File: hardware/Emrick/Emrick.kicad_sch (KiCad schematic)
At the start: 85 parts, among them J1 LED_STRIP_CONNECTOR, J2 UFL, J3 Conn_02x05_Odd_Even, J4 BATT_CONN, P1 USB_C_Plug_USB2.0, Q1 Q_NPN_DGS, Q2 Q_NPN_DGS, Q3 Q_NPN_DGS, SW1 SW_SPST, SW2 SW_MEC_5E (RESET), U1 74HCT541, U2 CC1310, U3 TPS63020, U4 CP2102N, U5 MX25R8035F, U6 BQ24072, Y1 24MHz, Y2 32.768kHz

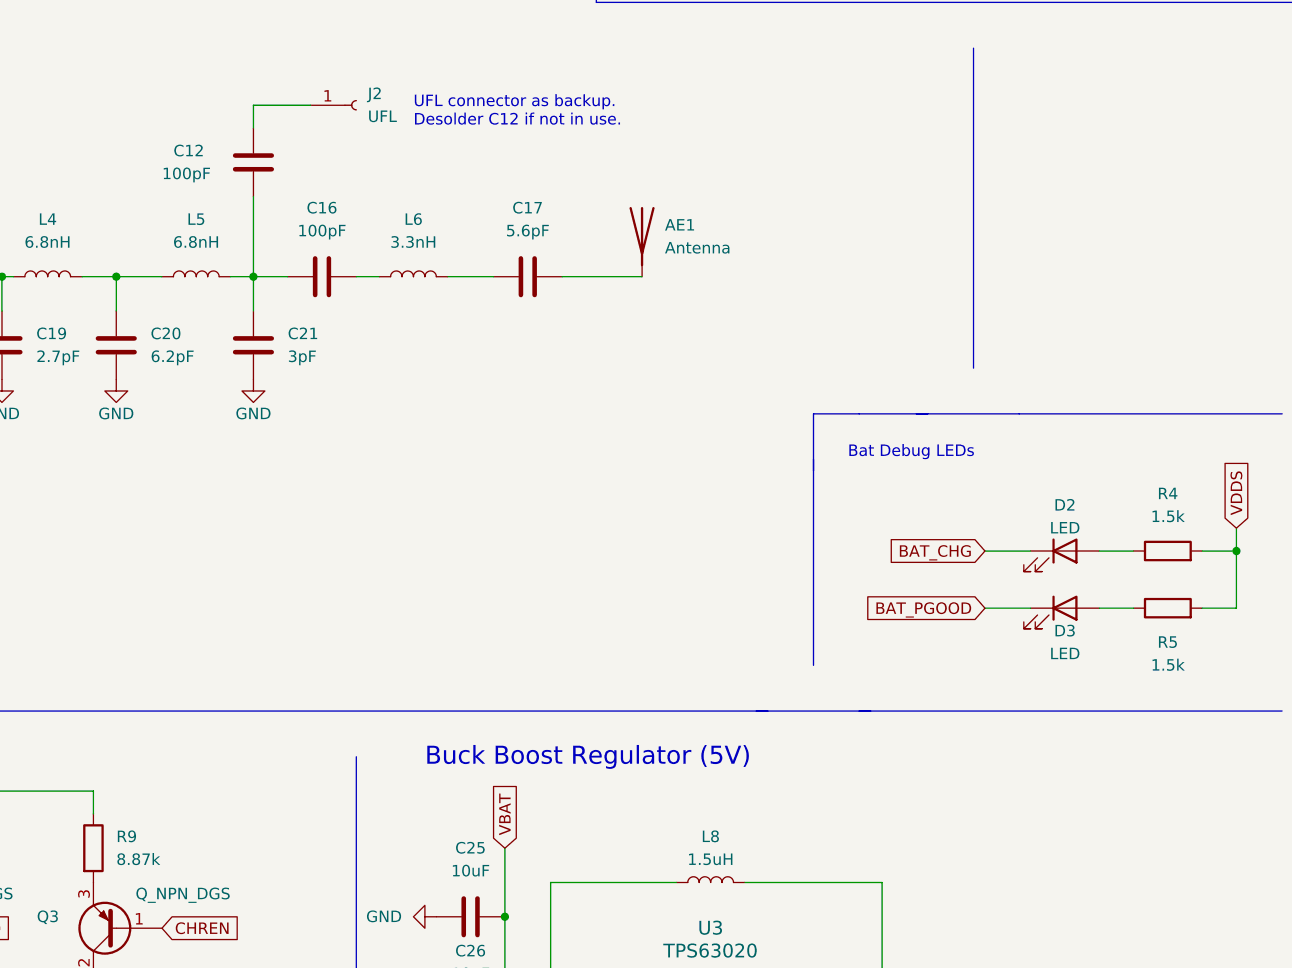
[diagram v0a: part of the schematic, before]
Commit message: some work on pcb and schematic
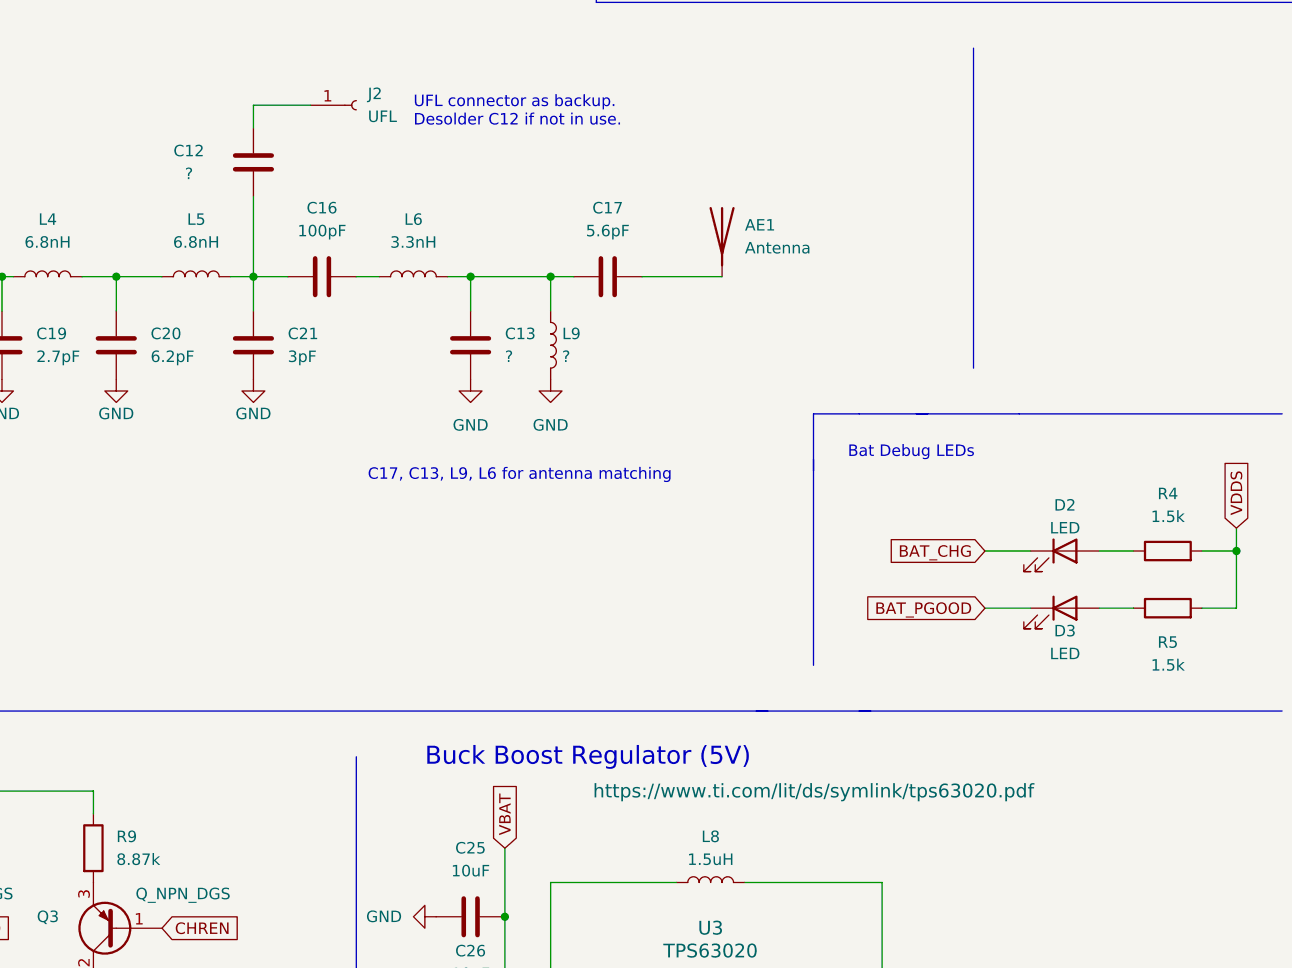
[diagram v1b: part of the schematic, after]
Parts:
- added C13: ?, Capacitor_SMD:C_0402_1005Metric, symbol Device:C
- added L9: ?, Inductor_SMD:L_0402_1005Metric, symbol Device:L
- C12: value 100pF -> ?
- SW1: footprint Connector_PinHeader_2.54mm:PinHeader_1x03_P2.54mm_Vertical -> switch:SW-TH_3P-P4.70_L11.1-W12.7
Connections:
- net GND: now also C13.2, L9.2
- net at C17.1, L6.2: now also C13.1, L9.1
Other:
- note added: "C17, C13, L9, L6 for antenna matching"
- moved on the sheet: AE1, C17
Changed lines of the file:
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@@
   (junction (at 130.81 93.98) (diameter 0) (color 0 0 0 0)
   )
+  (junction (at 311.15 118.11) (diameter 0) (color 0 0 0 0)
+  )
   (junction (at 118.11 93.98) (diameter 0) (color 0 0 0 0)
   )
@@
   (junction (at 240.03 121.92) (diameter 0) (color 0 0 0 0)
   )
+  (junction (at 320.04 118.11) (diameter 0) (color 0 0 0 0)
+  )
   (junction (at 232.41 114.3) (diameter 0) (color 0 0 0 0)
   )
@@
     (stroke (width 0) (type default) (color 0 0 0 0))
   )
+  (wire (pts (xy 320.04 118.11) (xy 322.58 118.11))
+    (stroke (width 0) (type default) (color 0 0 0 0))
+  )
   (wire (pts (xy 153.67 228.6) (xy 156.21 228.6))
     (stroke (width 0) (type default) (color 0 0 0 0))
@@
     (stroke (width 0) (type default) (color 0 0 0 0))
   )
+  (wire (pts (xy 320.04 121.92) (xy 320.04 118.11))
+    (stroke (width 0) (type default) (color 0 0 0 0))
+  )
   (wire (pts (xy 377.19 220.98) (xy 377.19 222.25))
     (stroke (width 0) (type default) (color 0 0 0 0))
@@
     (stroke (width 0) (type default) (color 0 0 0 0))
   )
+  (wire (pts (xy 311.15 121.92) (xy 311.15 118.11))
+    (stroke (width 0) (type default) (color 0 0 0 0))
+  )
   (wire (pts (xy 153.67 102.87) (xy 153.67 104.14))
     (stroke (width 0) (type default) (color 0 0 0 0))
@@
     (stroke (width 0) (type default) (color 0 0 0 0))
   )
-  (wire (pts (xy 308.61 118.11) (xy 313.69 118.11))
+  (wire (pts (xy 308.61 118.11) (xy 311.15 118.11))
     (stroke (width 0) (type default) (color 0 0 0 0))
   )
@@
     (stroke (width 0) (type default) (color 0 0 0 0))
   )
+  (wire (pts (xy 311.15 118.11) (xy 320.04 118.11))
+    (stroke (width 0) (type default) (color 0 0 0 0))
+  )
   (wire (pts (xy 365.76 215.9) (xy 365.76 219.71))
     (stroke (width 0) (type default) (color 0 0 0 0))
@@
     (stroke (width 0) (type default) (color 0 0 0 0))
   )
-  (wire (pts (xy 321.31 118.11) (xy 330.2 118.11))
+  (wire (pts (xy 330.2 118.11) (xy 339.09 118.11))
     (stroke (width 0) (type default) (color 0 0 0 0))
   )
@@
     (effects (font (size 2 2)) (justify left bottom))
   )
+  (text "C17, C13, L9, L6 for antenna matching" (at 299.72 140.97 0)
+    (effects (font (size 1.27 1.27)) (justify left bottom))
+  )
   (text "Programmable Power/Status LED\n" (at 85.09 20.32 0)
     (effects (font (size 1.27 1.27)) (justify left bottom))
@@
     (property "Reference" "SW1" (id 0) (at 90.17 187.96 0))
     (property "Value" "SW_SPST" (id 1) (at 88.9 190.5 0))
-    (property "Footprint" "Connector_PinHeader_2.54mm:PinHeader_1x03_P2.54mm_Vertical" (id 2) (at 102.87 185.42 0)
+    (property "Footprint" "switch:SW-TH_3P-P4.70_L11.1-W12.7" (id 2) (at 102.87 185.42 0)
       (effects (font (size 1.27 1.27)) hide)
     )
@@
     (pin "2")
   )
+  (symbol (lib_id "Device:L") (at 320.04 125.73 0) (unit 1)
+    (in_bom yes) (on_board yes) (fields_autoplaced)
+    (property "Reference" "L9" (id 0) (at 321.31 124.4599 0)
+      (effects (font (size 1.27 1.27)) (justify left))
+    )
+    (property "Value" "?" (id 1) (at 321.31 126.9999 0)
+      (effects (font (size 1.27 1.27)) (justify left))
+    )
+    (property "Footprint" "Inductor_SMD:L_0402_1005Metric" (id 2) (at 320.04 125.73 0)
+      (effects (font (size 1.27 1.27)) hide)
+    )
+    (property "Datasheet" "~" (id 3) (at 320.04 125.73 0)
+      (effects (font (size 1.27 1.27)) hide)
+    )
+    (pin "1")
+    (pin "2")
+  )
   (symbol (lib_id "power:GND") (at 151.13 274.32 0) (unit 1)
     (in_bom yes) (on_board yes) (fields_autoplaced)
@@
       (effects (font (size 1.27 1.27)) (justify left))
     )
-    (property "Value" "100pF" (id 1) (at 276.86 106.68 0)
+    (property "Value" "?" (id 1) (at 279.4 106.68 0)
       (effects (font (size 1.27 1.27)) (justify left))
     )
@@
     (pin "1")
   )
+  (symbol (lib_id "Device:C") (at 311.15 125.73 0) (unit 1)
+    (in_bom yes) (on_board yes) (fields_autoplaced)
+    (property "Reference" "C13" (id 0) (at 314.96 124.4599 0)
+      (effects (font (size 1.27 1.27)) (justify left))
+    )
+    (property "Value" "?" (id 1) (at 314.96 126.9999 0)
+      (effects (font (size 1.27 1.27)) (justify left))
+    )
+    (property "Footprint" "Capacitor_SMD:C_0402_1005Metric" (id 2) (at 312.1152 129.54 0)
+      (effects (font (size 1.27 1.27)) hide)
+    )
+    (property "Datasheet" "~" (id 3) (at 311.15 125.73 0)
+      (effects (font (size 1.27 1.27)) hide)
+    )
+    (pin "1")
+    (pin "2")
+  )
   (symbol (lib_id "Device:R") (at 284.48 255.27 90) (unit 1)
     (in_bom yes) (on_board yes)
@@
     (pin "1")
   )
-  (symbol (lib_id "Device:Antenna") (at 330.2 113.03 0) (unit 1)
+  (symbol (lib_id "Device:Antenna") (at 339.09 113.03 0) (unit 1)
     (in_bom yes) (on_board yes) (fields_autoplaced)
-    (property "Reference" "AE1" (id 0) (at 332.74 112.3949 0)
+    (property "Reference" "AE1" (id 0) (at 341.63 112.3949 0)
       (effects (font (size 1.27 1.27)) (justify left))
     )
-    (property "Value" "Antenna" (id 1) (at 332.74 114.9349 0)
+    (property "Value" "Antenna" (id 1) (at 341.63 114.9349 0)
       (effects (font (size 1.27 1.27)) (justify left))
     )
-    (property "Footprint" "Emrick Footprints:emrick_custom_antenna" (id 2) (at 330.2 113.03 0)
+    (property "Footprint" "Emrick Footprints:emrick_custom_antenna" (id 2) (at 339.09 113.03 0)
       (effects (font (size 1.27 1.27)) hide)
     )
-    (property "Datasheet" "~" (id 3) (at 330.2 113.03 0)
+    (property "Datasheet" "~" (id 3) (at 339.09 113.03 0)
       (effects (font (size 1.27 1.27)) hide)
     )
@@
       (effects (font (size 1.524 1.524)) hide)
     )
-    (property "Datasheet" "" (id 3) (at 356.87 218.44 0)
+    (property "Datasheet" "https://www.ti.com/lit/ds/symlink/tps63020.pdf" (id 3) (at 349.25 175.26 0)
       (effects (font (size 1.524 1.524)))
     )
@@
     (pin "2")
   )
-  (symbol (lib_id "Device:C") (at 317.5 118.11 90) (unit 1)
+  (symbol (lib_id "Device:C") (at 326.39 118.11 90) (unit 1)
     (in_bom yes) (on_board yes) (fields_autoplaced)
-    (property "Reference" "C17" (id 0) (at 317.5 110.49 90))
-    (property "Value" "5.6pF" (id 1) (at 317.5 113.03 90))
-    (property "Footprint" "Capacitor_SMD:C_0402_1005Metric" (id 2) (at 321.31 117.1448 0)
+    (property "Reference" "C17" (id 0) (at 326.39 110.49 90))
+    (property "Value" "5.6pF" (id 1) (at 326.39 113.03 90))
+    (property "Footprint" "Capacitor_SMD:C_0402_1005Metric" (id 2) (at 330.2 117.1448 0)
       (effects (font (size 1.27 1.27)) hide)
     )
-    (property "Datasheet" "~" (id 3) (at 317.5 118.11 0)
+    (property "Datasheet" "~" (id 3) (at 326.39 118.11 0)
       (effects (font (size 1.27 1.27)) hide)
     )
@@
     (pin "2")
   )
+  (symbol (lib_id "power:GND") (at 311.15 129.54 0) (unit 1)
+    (in_bom yes) (on_board yes) (fields_autoplaced)
+    (property "Reference" "#PWR016" (id 0) (at 311.15 135.89 0)
+      (effects (font (size 1.27 1.27)) hide)
+    )
+    (property "Value" "GND" (id 1) (at 311.15 134.62 0))
+    (property "Footprint" "" (id 2) (at 311.15 129.54 0)
+      (effects (font (size 1.27 1.27)) hide)
+    )
+    (property "Datasheet" "" (id 3) (at 311.15 129.54 0)
+      (effects (font (size 1.27 1.27)) hide)
+    )
+    (pin "1")
+  )
   (symbol (lib_id "Device:C") (at 259.08 125.73 0) (unit 1)
     (in_bom yes) (on_board yes) (fields_autoplaced)
@@
     (pin "1")
   )
+  (symbol (lib_id "power:GND") (at 320.04 129.54 0) (unit 1)
+    (in_bom yes) (on_board yes) (fields_autoplaced)
+    (property "Reference" "#PWR049" (id 0) (at 320.04 135.89 0)
+      (effects (font (size 1.27 1.27)) hide)
+    )
+    (property "Value" "GND" (id 1) (at 320.04 134.62 0))
+    (property "Footprint" "" (id 2) (at 320.04 129.54 0)
+      (effects (font (size 1.27 1.27)) hide)
+    )
+    (property "Datasheet" "" (id 3) (at 320.04 129.54 0)
+      (effects (font (size 1.27 1.27)) hide)
+    )
+    (pin "1")
+  )
   (symbol (lib_id "Device:R") (at 31.75 238.76 0) (unit 1)
     (in_bom yes) (on_board yes) (fields_autoplaced)
@@
       (reference "#PWR015") (unit 1) (value "GND") (footprint "")
     )
+    (path "/c4a0c265-4b39-41d3-ab53-2ab4874fa3fe"
+      (reference "#PWR016") (unit 1) (value "GND") (footprint "")
+    )
     (path "/1114404f-4690-4e3f-9b08-e30201bf3fb3"
       (reference "#PWR017") (unit 1) (value "GND") (footprint "")
@@
       (reference "#PWR048") (unit 1) (value "GND") (footprint "")
     )
+    (path "/eaf0c0f4-f8ef-48ee-830b-828643b639bd"
+      (reference "#PWR049") (unit 1) (value "GND") (footprint "")
+    )
     (path "/d7b546ac-1aeb-4e32-be9e-b8ba6b0d2d70"
       (reference "#PWR050") (unit 1) (value "GND") (footprint "")
@@
     )
     (path "/4f3938ec-ee10-4033-b043-17e527f7cafe"
-      (reference "C12") (unit 1) (value "100pF") (footprint "Capacitor_SMD:C_0402_1005Metric")
+      (reference "C12") (unit 1) (value "?") (footprint "Capacitor_SMD:C_0402_1005Metric")
+    )
+    (path "/50c8f597-eecd-41b3-b369-057fd39f4039"
+      (reference "C13") (unit 1) (value "?") (footprint "Capacitor_SMD:C_0402_1005Metric")
     )
     (path "/131a06d2-a108-46d7-83da-eec9c5e5b8d7"
@@
       (reference "L8") (unit 1) (value "1.5uH") (footprint "Inductor_SMD:L_Sunlord_MWSA0518_5.4x5.2mm")
     )
+    (path "/3240c5b7-b3f1-4039-96ce-b8816fd0780e"
+      (reference "L9") (unit 1) (value "?") (footprint "Inductor_SMD:L_0402_1005Metric")
+    )
     (path "/98b2397c-2d8e-4422-bb18-42d4b4daae2e"
       (reference "P1") (unit 1) (value "USB_C_Plug_USB2.0") (footprint "Connector_USB:USB_C_Receptacle_XKB_U262-16XN-4BVC11")
@@
     )
     (path "/296a890d-93e3-479a-910f-fa1bd31332ae"
-      (reference "SW1") (unit 1) (value "SW_SPST") (footprint "Connector_PinHeader_2.54mm:PinHeader_1x03_P2.54mm_Vertical")
+      (reference "SW1") (unit 1) (value "SW_SPST") (footprint "switch:SW-TH_3P-P4.70_L11.1-W12.7")
     )
     (path "/b30242dc-8228-402b-8e4f-fd03a02393d4"
